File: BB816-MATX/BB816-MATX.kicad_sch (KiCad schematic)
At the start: 17 parts, among them J1 10018783-10113TLF, J2 10018783-10113TLF, J3 10018783-10113TLF, J4 10018783-10113TLF, J5 39-28-1243, J6 PinSocket_2x40_P2.54mm_Vertic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, J7 PinSocket_1x02_P2.54mm_Vertic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, J8 PinSocket_2x18_P2.54mm_Vertic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

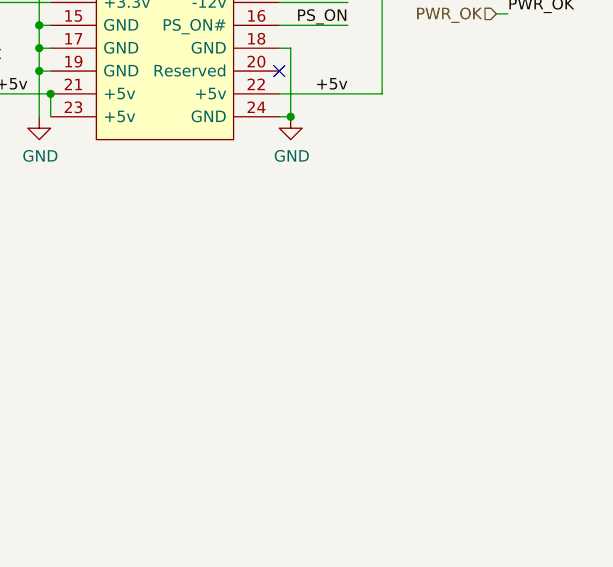
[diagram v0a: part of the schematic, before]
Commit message: doc
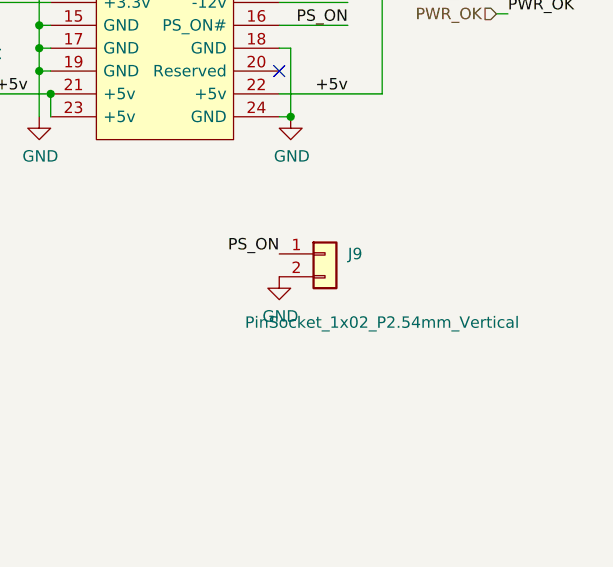
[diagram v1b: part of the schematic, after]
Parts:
- added J9: PinSocket_1x02_P2.54mm_Vertical, Connector_PinSocket_2.54mm:PinSocket_1x02_P2.54mm_Vertical, symbol BB816-MATX-PCIE:PinSocket_1x02_P2.54mm_Vertical
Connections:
- net GND: now also J9.2 (Pin_2)
- net PS_ON: now also J9.1 (Pin_1)
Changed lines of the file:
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@@
     (effects (font (size 1.27 1.27)) (justify left bottom))
+  )
+  (label "PS_ON" (at 363.22 68.58 180) (fields_autoplaced)
+    (effects (font (size 1.27 1.27)) (justify right bottom))
   )
   (label "A15" (at 81.28 111.76 0) (fields_autoplaced)
@@
     )
   )
+  (symbol (lib_id "CM4_MATX:GND") (at 363.22 71.12 0) (unit 1)
+    (in_bom yes) (on_board yes) (dnp no)
+    (property "Reference" "#PWR012" (at 363.22 77.47 0)
+      (effects (font (size 1.27 1.27)) hide)
+    )
+    (property "Value" "GND" (at 363.347 75.5142 0)
+      (effects (font (size 1.27 1.27)))
+    )
+    (property "Footprint" "" (at 363.22 71.12 0)
+      (effects (font (size 1.27 1.27)) hide)
+    )
+    (property "Datasheet" "" (at 363.22 71.12 0)
+      (effects (font (size 1.27 1.27)) hide)
+    )
+    (pin "1")
+    (instances
+      (project "BB816-MATX"
+        (path "/e71bf3dc-e3a5-46de-b13d-86fbd18272fb"
+          (reference "#PWR012") (unit 1)
+        )
+      )
+    )
+  )
   (symbol (lib_id "BB816-MATX-PCIE:10018783-10113TLF") (at 116.84 25.4 0) (mirror y) (unit 1)
     (in_bom yes) (on_board yes) (dnp no)
@@
         )
       )
+    )
+  )
+  (symbol (lib_id "BB816-MATX-PCIE:PinSocket_1x02_P2.54mm_Vertical") (at 368.3 68.58 0) (unit 1)
+    (in_bom yes) (on_board yes) (dnp no)
+    (property "Reference" "J9" (at 370.84 68.58 0)
+      (effects (font (size 1.27 1.27)) (justify left))
+    )
+    (property "Value" "PinSocket_1x02_P2.54mm_Vertical" (at 359.41 76.2 0)
+      (effects (font (size 1.27 1.27)) (justify left))
+    )
+    (property "Footprint" "Connector_PinSocket_2.54mm:PinSocket_1x02_P2.54mm_Vertical" (at 368.3 68.58 0)
+      (effects (font (size 1.27 1.27)) hide)
+    )
+    (property "Datasheet" "~" (at 368.3 68.58 0)
+      (effects (font (size 1.27 1.27)) hide)
+    )
+    (pin "1")
+    (pin "2")
+    (instances
+      (project "BB816-MATX"
+        (path "/e71bf3dc-e3a5-46de-b13d-86fbd18272fb"
+          (reference "J9") (unit 1)
+        )
+      )

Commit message: BankZero
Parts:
- added C1, C2, C3, C4, C5, C6, C7: 220u, Capacitor_THT:CP_Radial_D6.3mm_P2.50mm, symbol Device:C_Polarized_Small
- added J10: BB816_Breakout_A27, BB816-MATX-PCIE:BB816_Breakout_A27_Socket_NO_VDPA, symbol BB816-MATX-PCIE:BB816_Breakout_A27_Socket
- added J11: PinSocket_1x02_P2.54mm_Vertical, Connector_PinSocket_2.54mm:PinSocket_1x02_P2.54mm_Vertical, symbol BB816-MATX-PCIE:PinSocket_1x02_P2.54mm_Vertical
- J9: value PinSocket_1x02_P2.54mm_Vertical -> PWR_SW
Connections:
- net A0: now also J10.b50 (A0)
- net A1: now also J10.b49 (A1)
- net A10: now also J10.b40 (A10)
- net A11: now also J10.b39 (A11)
- net A12: now also J10.b38 (A12)
- net A13: now also J10.b37 (A13)
- net A14: now also J10.b36 (A14)
- net A15: now also J10.b35 (A15)
- net A16: now also J10.b34 (A16)
- net A17: now also J10.b33 (A17)
- net A18: now also J10.b32 (A18)
- net A19: now also J10.b31 (A19)
- net A2: now also J10.b48 (A2)
- net A20: now also J10.b30 (A20)
- net A21: now also J10.b29 (A21)
- net A22: now also J10.b28 (A22)
- net A23: now also J10.b27 (A23)
- net A3: now also J10.b47 (A3)
- net A4: now also J10.b46 (A4)
- net A5: now also J10.b45 (A5)
- net A6: now also J10.b44 (A6)
- net A7: now also J10.b43 (A7)
- net A8: now also J10.b42 (A8)
- net A9: now also J10.b41 (A9)
- net BE: now also J10.b13 (BE)
- net CLK: now also J10.b8 (CLK)
- net CLK_SRC: now also J10.b7 (CLK_SRC)
- net D0: now also J10.b58 (D0)
- net D1: now also J10.b57 (D1)
- net D2: now also J10.b56 (D2)
- net D3: now also J10.b55 (D3)
- net D4: now also J10.b54 (D4)
- net D5: now also J10.b53 (D5)
- net D6: now also J10.b52 (D6)
- net D7: now also J10.b51 (D7)
- net E: now also J10.b22 (E)
- net GND: now also C1.2, C2.2, C3.2, C4.2, C5.2, C6.2, C7.2, J10.a10 (GND), J10.a11 (GND), J10.a12 (GND), J10.a13 (GND), J10.a14 (GND), J10.a15 (GND), J10.a16 (GND), J10.a17 (GND), J10.a18 (GND), J10.a19 (GND), J10.a2 (GND), J10.a20 (GND), J10.a21 (GND), J10.a22 (GND), J10.a23 (GND), J10.a24 (GND), J10.a25 (GND), J10.a26 (GND), J10.a27 (GND), J10.a28 (GND), J10.a29 (GND), J10.a3 (GND), J10.a30 (GND), J10.a31 (GND), J10.a32 (GND), J10.a33 (GND), J10.a34 (GND), J10.a35 (GND), J10.a36 (GND), J10.a37 (GND), J10.a38 (GND), J10.a39 (GND), J10.a4 (GND), J10.a40 (GND), J10.a41 (GND), J10.a42 (GND), J10.a43 (GND), J10.a44 (GND), J10.a45 (GND), J10.a46 (GND), J10.a47 (GND), J10.a48 (GND), J10.a49 (GND), J10.a5 (GND), J10.a50 (GND), J10.a51 (GND), J10.a52 (GND), J10.a53 (GND), J10.a54 (GND), J10.a55 (GND), J10.a56 (GND), J10.a57 (GND), J10.a58 (GND), J10.a6 (GND), J10.a7 (GND), J10.a8 (GND), J10.a9 (GND), J10.b2 (GND)
- net M: now also J10.b23 (M)
- net RDY_IN: now also J10.b14 (RDY_IN)
- net RST: now also J10.b5 (RST)
- net R~{W}: now also J10.b18 (R~{W})
- net SYNC: now also J10.b16 (SYNC)
- net VA: now also J10.b17 (VA)
- net VCC: now also C1.1, C2.1, C3.1, C4.1, C5.1, C6.1, C7.1, J10.b1 (VCC)
- net VDA: now also J11.1 (Pin_1)
- net VPA: now also J11.2 (Pin_2)
- net X: now also J10.b24 (X)
- net ~{ABORT}: now also J10.b12 (~{ABORT})
- net ~{BANK0}: now also J10.b21 (~{BANK0})
- net ~{CLK_EN}: now also J10.b6 (~{CLK_EN})
- net ~{CLK}: now also J10.b9 (~{CLK})
- net ~{IRQ}: now also J10.b10 (~{IRQ})
- net ~{ML}: now also J10.b26 (~{ML})
- net ~{MR}⎒: now also J10.b3 (~{MR}⎒)
- net ~{NMI}: now also J10.b11 (~{NMI})
- net ~{RD}: now also J10.b19 (~{RD})
- net ~{RST}: now also J10.b4 (~{RST})
- net ~{VP}: now also J10.b25 (~{VP})
- net ~{WAI}: now also J10.b15 (~{WAI})
- net ~{WR}: now also J10.b20 (~{WR})
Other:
- added sheet BB816_BankZero (BB816_BankZero.kicad_sch)
- moved on the sheet: J1, J2, J3, J4, J6, J7, J8, J9
